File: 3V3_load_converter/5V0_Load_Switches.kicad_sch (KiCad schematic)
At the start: 29 parts, among them Q21 SI2302DDS-T1-GE3, Q22 SI2302DDS-T1-GE3, Q23 SI2302DDS-T1-GE3, U10 INA199C3DCKR, U11 LMV321RIYLT, U12 NVTFS5116PLTAG, U13 NVTFS5116PLTAG, U14 NVTFS5116PLTAG, U8 INA199C1DCKR, U9 INA199C3DCKR

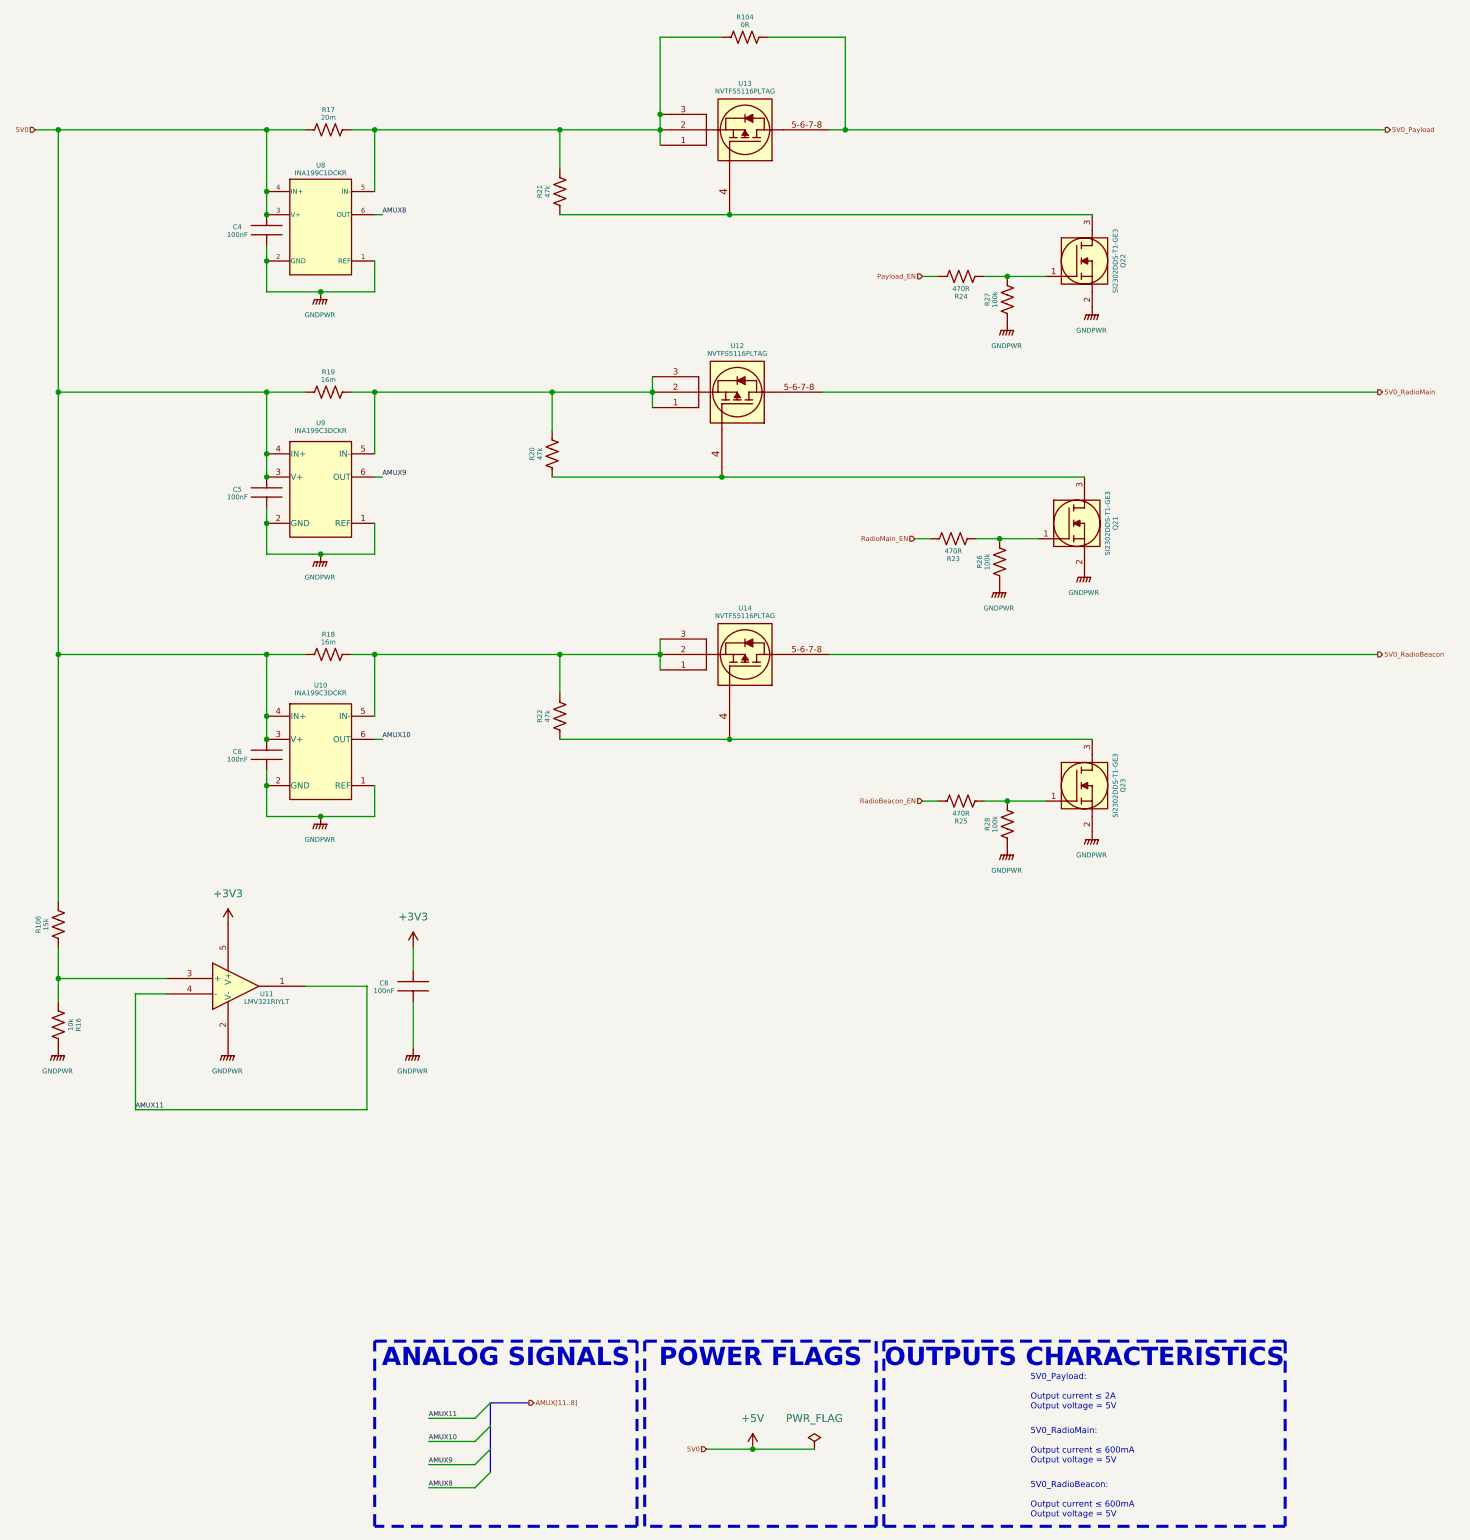
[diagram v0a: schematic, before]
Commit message: update
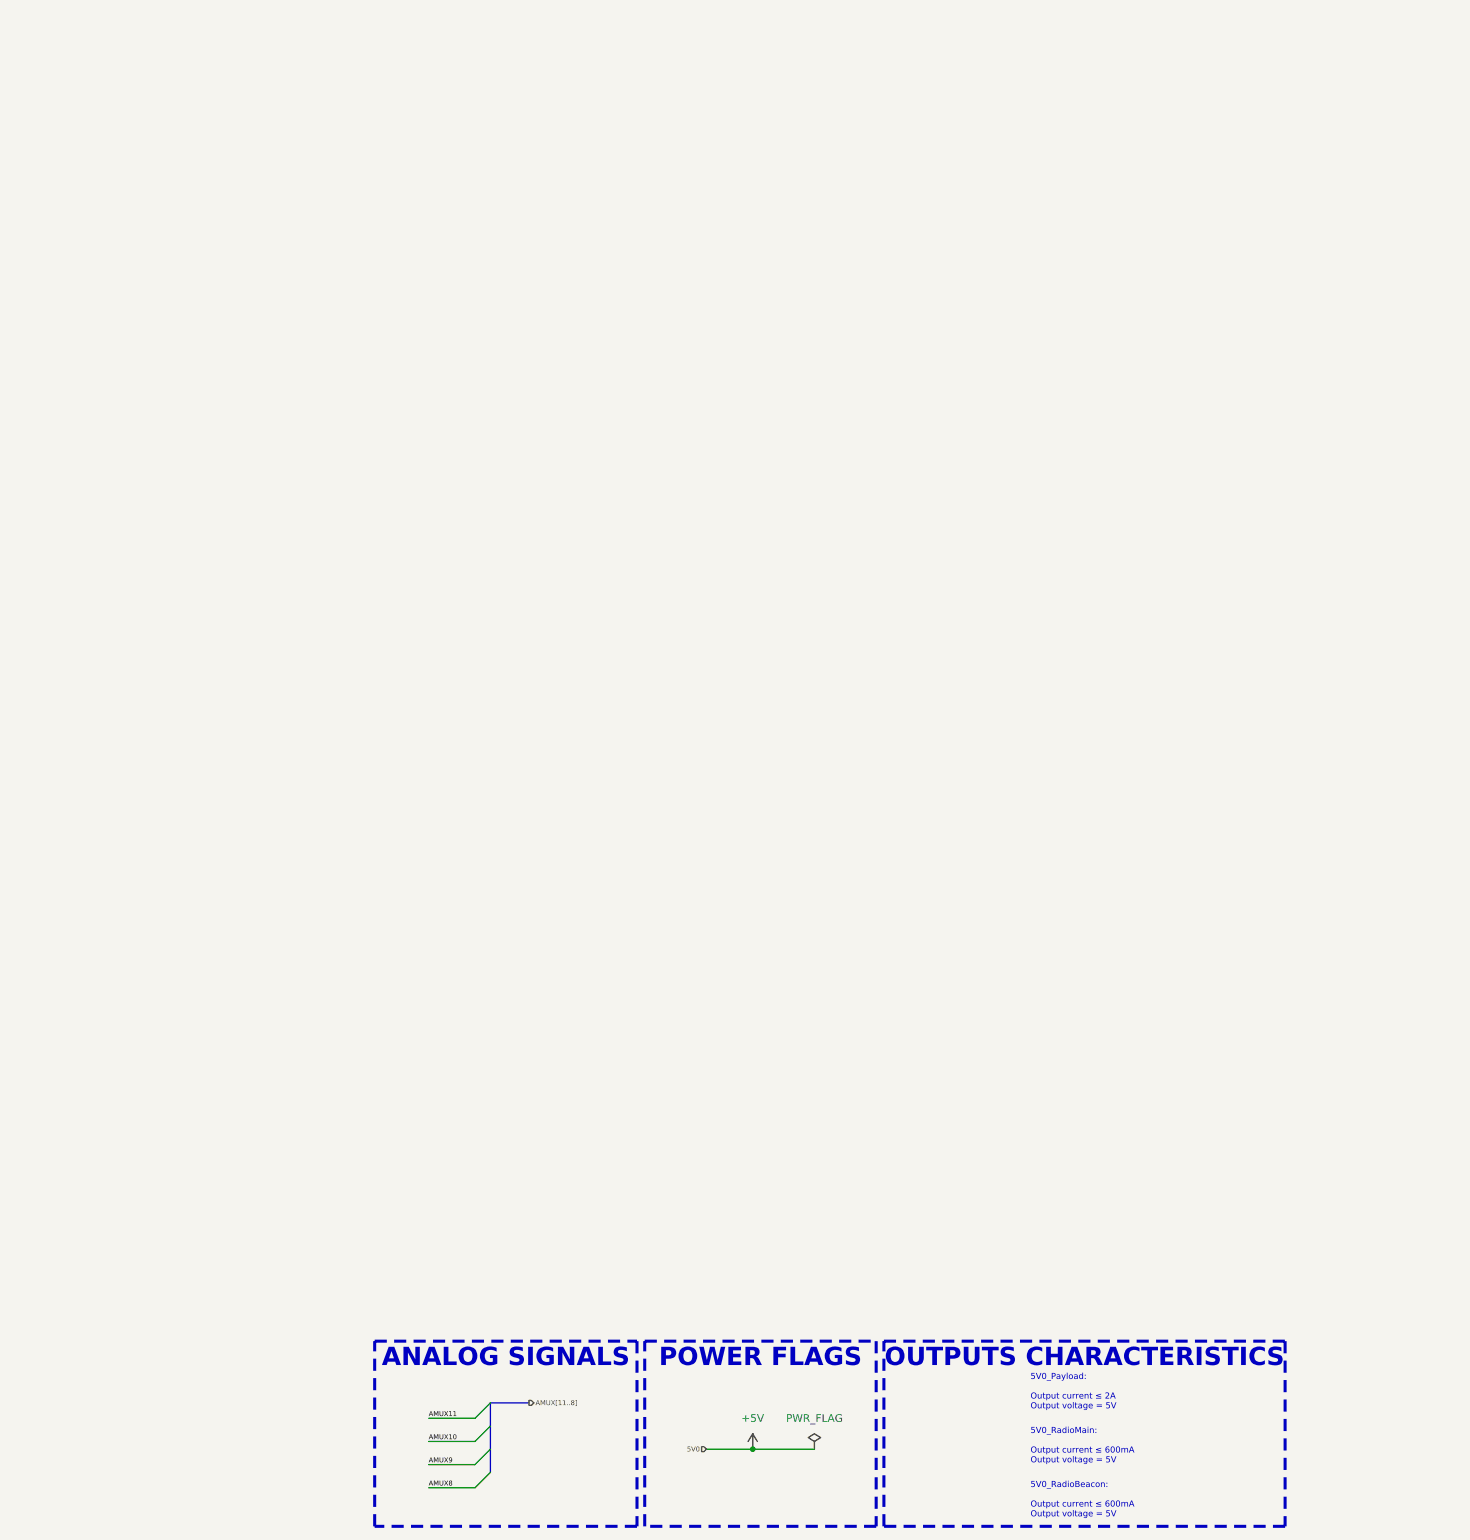
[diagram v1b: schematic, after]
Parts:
- removed C4, C5, C6, C8: 100nF, footprints:CAP0603, symbol C0603C104K5RACTU:C0603C104K5RACTU
- removed Q21, Q22, Q23: SI2302DDS-T1-GE3, footprints:SI2302DDS-T1-GE3, symbol SI2302DDS-T1-GE3:SI2302DDS-T1-GE3
- removed R104: 0R, footprints:RES0603, symbol CRCW06030000Z0EAHP:CRCW06030000Z0EAHP
- removed R106: 15k, footprints:RES0603, symbol CRCW060315K0FKEAHP:CRCW060315K0FKEAHP
- removed R16: 10k, footprints:RES0805, symbol RC0805FR-0710KL:RC0805FR-0710KL
- removed R17: 20m, footprints:RES2010, symbol WSL2010R0200FEA:WSL2010R0200FEA
- removed R18, R19: 16m, footprints:RES2010, symbol WSL2010R0160FEA:WSL2010R0160FEA
- removed R20, R21, R22: 47k, footprints:RES0603, symbol CRCW060347K0FKEAHP:CRCW060347K0FKEAHP
- removed R23, R24, R25: 470R, footprints:RES0603, symbol CRCW0603470RFKEAHP:CRCW0603470RFKEAHP
- removed R26, R27, R28: 100k, footprints:RES0603, symbol CRCW0603100KFKEAHP:CRCW0603100KFKEAHP
- removed U10, U9: INA199C3DCKR, footprints:INA199C3DCKR, symbol INA199C3DCKR:INA199C3DCKR
- removed U11: LMV321RIYLT, footprints:LMV321RIYLT, symbol LMV321RIYLT:LMV321RIYLT
- removed U12, U13, U14: NVTFS5116PLTAG, footprints:NVTFS5116PLTAG, symbol NVTFS5116PLWFTAG:NVTFS5116PLTAG
- removed U8: INA199C1DCKR, footprints:INA199C1DCKR, symbol INA199C1DCKR:INA199C1DCKR
